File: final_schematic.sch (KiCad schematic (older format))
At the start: 49 parts, among them J1 Battery Babysitter, J2 BB_SYSOFF, J3 BOOT0, J4 OLED Qwiic, J5 Programmer, J8 GPS_COAX, SW1 SW_Push_SESS, SW2 SW_Push_RADIO, SW3 SW_Push_RST, U1 STM32L476VGTx, U2 MTK3339, U3 RFM95W-868S2, U4 BNO055, U5 LT1129-3.3_SO8

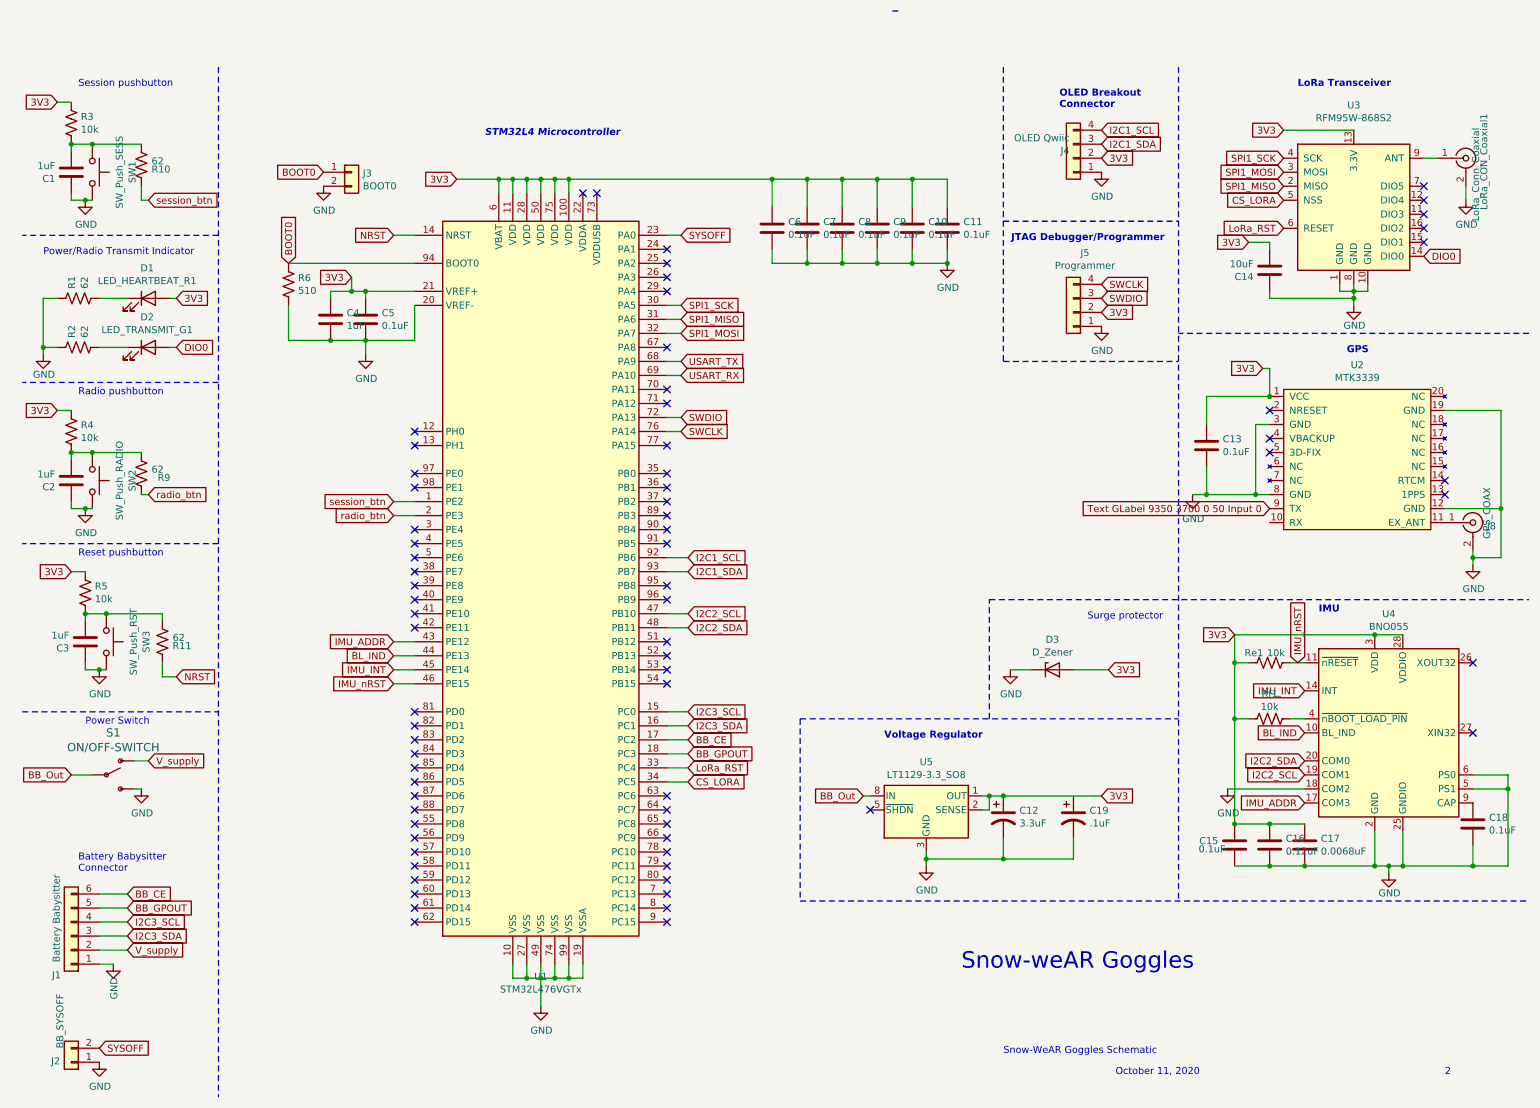
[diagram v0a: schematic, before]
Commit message: Schematic FINAL 	modified:   final_schematic-cache.lib 	modified:   final_schematic.sch 	modified:   final_schematic.sch-bak
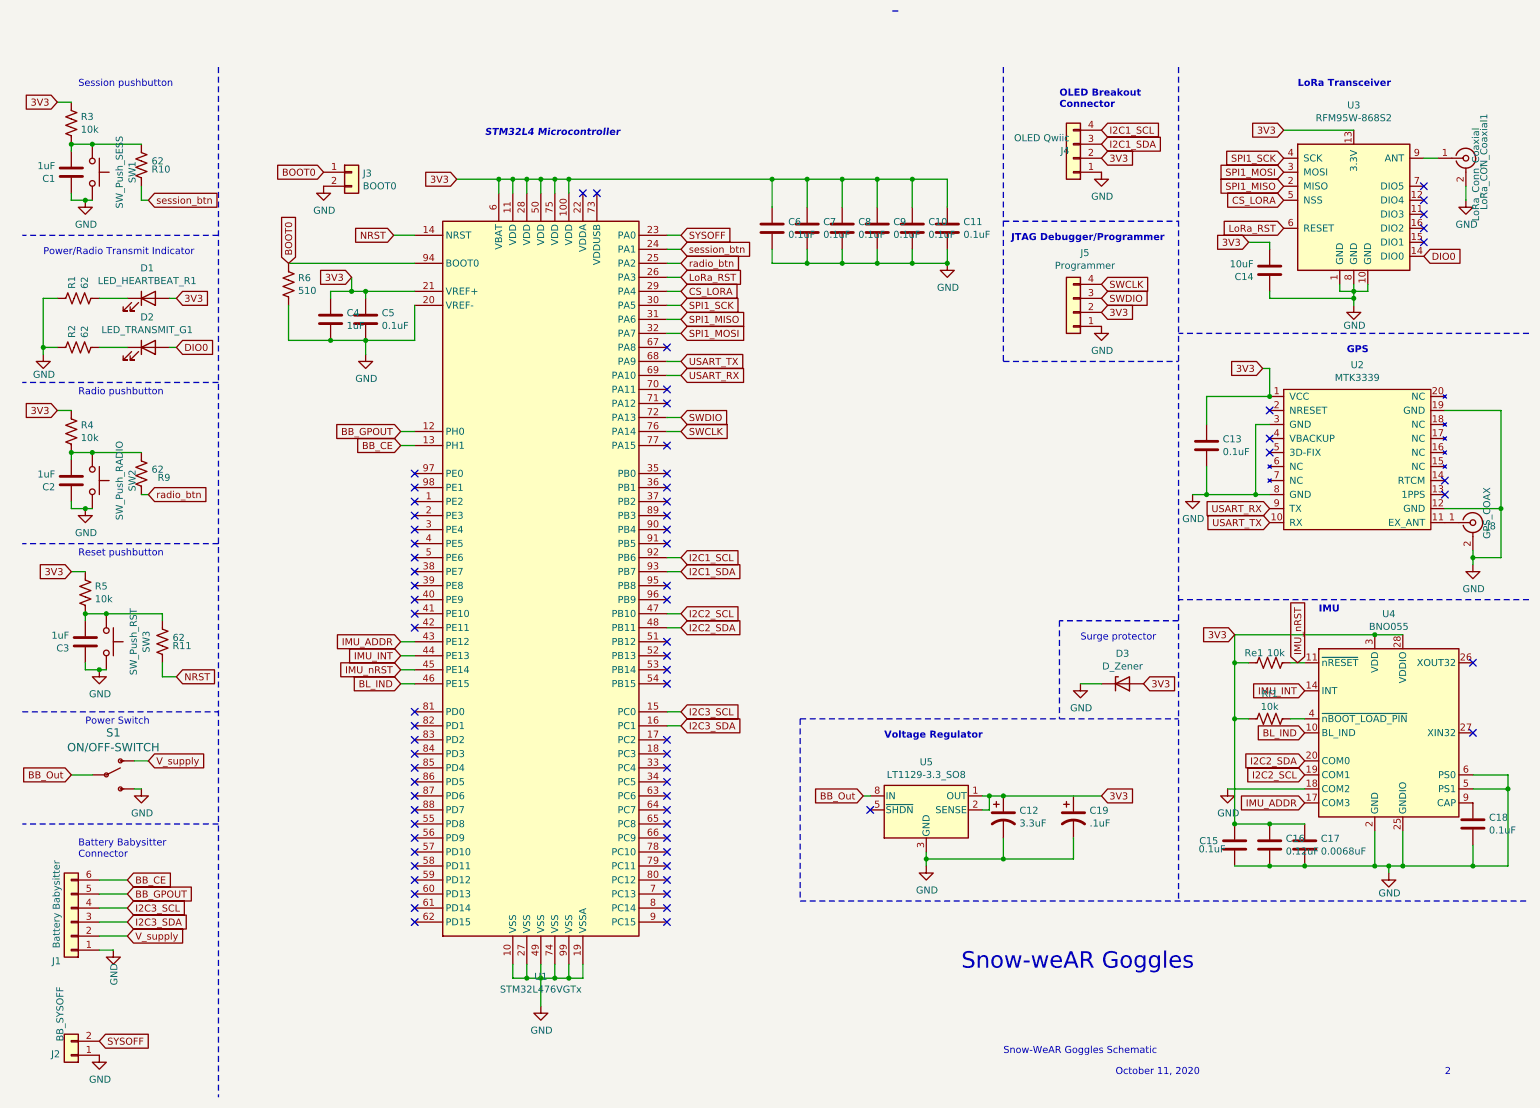
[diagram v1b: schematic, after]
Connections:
- net Text GLabel 9350 3700 0    50   Input ~ 0 is gone; now on net USART_RX: U2.9 (TX)
- net BB_CE: now also U1.13 (PH1); no longer U1.17 (PC2)
- net BB_GPOUT: now also U1.12 (PH0); no longer U1.18 (PC3)
- net BL_IND: now also U1.46 (PE15); no longer U1.44 (PE13)
- net CS_LORA: now also U1.29 (PA4); no longer U1.34 (PC5)
- net IMU_INT: now also U1.44 (PE13); no longer U1.45 (PE14)
- net IMU_nRST: now also U1.45 (PE14); no longer U1.46 (PE15)
- net LoRa_RST: now also U1.26 (PA3); no longer U1.33 (PC4)
- net USART_TX: now also U2.10 (RX)
- net radio_btn: now also U1.25 (PA2); no longer U1.2 (PE3)
- net session_btn: now also U1.24 (PA1); no longer U1.1 (PE2)
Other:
- moved on the sheet: D3, J1, J2
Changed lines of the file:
@@
 EESchema Schematic File Version 4
-LIBS:final_schematic-cache
-EELAYER 26 0
+EELAYER 30 0
 EELAYER END
 $Descr A4 11693 8268
@@
 $EndComp
 Text GLabel 9350 3600 0    50   Input ~ 0
-Text GLabel 9350 3700 0    50   Input ~ 0
-USART_TX
+USART_RX
 $Comp
 L final_schematic-rescue:MTK3339-GPS-rescue U2
@@
 L Connector_Generic:Conn_01x06 J1
 U 1 1 5FF26B1F
-P 800 6650
-F 0 "J1" H 906 6928 50  0000 C CNN
-F 1 "Battery Babysitter" V 906 6837 50  0000 R CNN
-F 2 "Connector_PinHeader_1.00mm:PinHeader_1x06_P1.00mm_Vertical" H 800 6650 50  0001 C CNN
-F 3 "~" H 800 6650 50  0001 C CNN
-	1    800  6650
+P 800 6550
+F 0 "J1" H 906 6828 50  0000 C CNN
+F 1 "Battery Babysitter" V 906 6737 50  0000 R CNN
+F 2 "Connector_PinHeader_1.00mm:PinHeader_1x06_P1.00mm_Vertical" H 800 6550 50  0001 C CNN
+F 3 "~" H 800 6550 50  0001 C CNN
+	1    800  6550
 	-1   0    0    1
 $EndComp
-Text Notes 850  6200 0    50   ~ 0
+Text Notes 850  6100 0    50   ~ 0
 Battery Babysitter \nConnector
+Text GLabel 1200 6550 2    50   Input ~ 0
+I2C3_SDA
+Text GLabel 1200 6450 2    50   Input ~ 0
+I2C3_SCL
 Text GLabel 1200 6650 2    50   Input ~ 0
-I2C3_SDA
-Text GLabel 1200 6550 2    50   Input ~ 0
-I2C3_SCL
-Text GLabel 1200 6750 2    50   Input ~ 0
 V_supply
 Wire Wire Line
-	1200 6750 1000 6750
-Wire Wire Line
 	1200 6650 1000 6650
+Wire Wire Line
+	1200 6550 1000 6550
 $Comp
 L power:GND #PWR05
 U 1 1 60007EB3
-P 1100 6850
-F 0 "#PWR05" H 1100 6600 50  0001 C CNN
-F 1 "GND" V 1105 6677 50  0000 C CNN
-F 2 "" H 1100 6850 50  0001 C CNN
-F 3 "" H 1100 6850 50  0001 C CNN
-	1    1100 6850
-	1    0    0    -1
-$EndComp
-Wire Wire Line
-	1200 6550 1000 6550
+P 1100 6750
+F 0 "#PWR05" H 1100 6500 50  0001 C CNN
+F 1 "GND" V 1105 6577 50  0000 C CNN
+F 2 "" H 1100 6750 50  0001 C CNN
+F 3 "" H 1100 6750 50  0001 C CNN
+	1    1100 6750
+	1    0    0    -1
+$EndComp
+Wire Wire Line
+	1200 6450 1000 6450
 Text Notes 8600 1700 2    50   ~ 10
 JTAG Debugger/Programmer
@@
 Text GLabel 9600 5500 0    50   Input ~ 0
 I2C2_SCL
-Text GLabel 1200 6450 2    50   Input ~ 0
+Text GLabel 1200 6350 2    50   Input ~ 0
 BB_GPOUT
 Wire Wire Line
-	1000 6350 1200 6350
-Wire Wire Line
-	1200 6450 1000 6450
+	1000 6250 1200 6250
+Wire Wire Line
+	1200 6350 1000 6350
 NoConn ~ 10600 3400
 NoConn ~ 10600 3500
@@
 Text GLabel 2800 1950 0    50   Input ~ 0
 3V3
-Text GLabel 3100 4650 0    50   Input ~ 0
+Text GLabel 3150 4850 0    50   Input ~ 0
 BL_IND
-Text GLabel 3100 4550 0    50   Input ~ 0
+Text GLabel 3150 4550 0    50   Input ~ 0
 IMU_ADDR
 Text GLabel 2600 1200 0    50   Input ~ 0
@@
 Text GLabel 5150 1650 2    50   Input ~ 0
 SYSOFF
-Text GLabel 5200 5350 2    50   Input ~ 0
+Text GLabel 3150 3050 0    50   Input ~ 0
 BB_GPOUT
-Text GLabel 3100 4850 0    50   Input ~ 0
+Text GLabel 3150 4750 0    50   Input ~ 0
 IMU_nRST
 NoConn ~ 3250 3450
@@
 NoConn ~ 5050 2850
 NoConn ~ 5050 2750
-NoConn ~ 5050 1850
-NoConn ~ 5050 1750
 NoConn ~ 4550 1350
 NoConn ~ 4450 1350
@@
 NoConn ~ 3250 3850
 NoConn ~ 3250 3750
-Text GLabel 3100 3550 0    50   Input ~ 0
+Text GLabel 5150 1750 2    50   Input ~ 0
 session_btn
-Text GLabel 3100 3650 0    50   Input ~ 0
+Text GLabel 5150 1850 2    50   Input ~ 0
 radio_btn
 Wire Wire Line
@@
 	4250 1250 4350 1250
 Connection ~ 4150 1250
-Text GLabel 3100 4750 0    50   Input ~ 0
+Text GLabel 3150 4650 0    50   Input ~ 0
 IMU_INT
-Text GLabel 5200 5550 2    50   Input ~ 0
+Text GLabel 5150 2050 2    50   Input ~ 0
 CS_LORA
-Text GLabel 5200 5450 2    50   Input ~ 0
+Text GLabel 5150 1950 2    50   Input ~ 0
 LoRa_RST
-Text GLabel 5200 5250 2    50   Input ~ 0
+Text GLabel 3150 3150 0    50   Input ~ 0
 BB_CE
-Text GLabel 5200 4450 2    50   Input ~ 0
+Text GLabel 5150 4450 2    50   Input ~ 0
 I2C2_SDA
-Text GLabel 5200 4350 2    50   Input ~ 0
+Text GLabel 5150 4350 2    50   Input ~ 0
 I2C2_SCL
 Connection ~ 4350 6950
@@
 Wire Wire Line
 	9050 5600 9600 5600
-Text GLabel 1200 6350 2    50   Input ~ 0
+Text GLabel 1200 6250 2    50   Input ~ 0
 BB_CE
 Wire Wire Line
@@
 L Connector_Generic:Conn_01x02 J2
 U 1 1 5FC7E508
-P 800 7550
-F 0 "J2" H 880 7542 50  0000 L CNN
-F 1 "BB_SYSOFF" V 880 7451 50  0000 R CNN
-F 2 "Connector_PinHeader_1.00mm:PinHeader_1x02_P1.00mm_Vertical" H 800 7550 50  0001 C CNN
-F 3 "~" H 800 7550 50  0001 C CNN
-	1    800  7550
+P 800 7500
+F 0 "J2" H 880 7492 50  0000 L CNN
+F 1 "BB_SYSOFF" V 880 7401 50  0000 R CNN
+F 2 "Connector_PinHeader_1.00mm:PinHeader_1x02_P1.00mm_Vertical" H 800 7500 50  0001 C CNN
+F 3 "~" H 800 7500 50  0001 C CNN
+	1    800  7500
 	-1   0    0    1
 $EndComp
@@
 L power:GND #PWR?
 U 1 1 5FC7E50E
-P 1000 7550
+P 1000 7500
 AR Path="/5F775B0B/5FC7E50E" Ref="#PWR?"  Part="1"
 AR Path="/5FC7E50E" Ref="#PWR0104"  Part="1"
-F 0 "#PWR0104" H 1000 7300 50  0001 C CNN
-F 1 "GND" H 1005 7377 50  0000 C CNN
-F 2 "" H 1000 7550 50  0001 C CNN
-F 3 "" H 1000 7550 50  0001 C CNN
-	1    1000 7550
-	1    0    0    -1
-$EndComp
-Text GLabel 1000 7450 2    50   Input ~ 0
+F 0 "#PWR0104" H 1000 7250 50  0001 C CNN
+F 1 "GND" H 1005 7327 50  0000 C CNN
+F 2 "" H 1000 7500 50  0001 C CNN
+F 3 "" H 1000 7500 50  0001 C CNN
+	1    1000 7500
+	1    0    0    -1
+$EndComp
+Text GLabel 1000 7400 2    50   Input ~ 0
 SYSOFF
 $Comp
@@
 NoConn ~ 6500 5750
 NoConn ~ 9350 3200
-NoConn ~ 5050 2050
 NoConn ~ 5050 2450
 NoConn ~ 5050 3650
 Wire Wire Line
-	1100 6850 1000 6850
+	1100 6750 1000 6750
 Wire Wire Line
 	7300 5750 7350 5750
@@
 	600  2450 600  2500
 Connection ~ 600  2450
-Text GLabel 5200 4050 2    50   Input ~ 0
+Text GLabel 5150 4050 2    50   Input ~ 0
 I2C1_SDA
-Text GLabel 5200 3950 2    50   Input ~ 0
+Text GLabel 5150 3950 2    50   Input ~ 0
 I2C1_SCL
-Text GLabel 5200 5150 2    50   Input ~ 0
+Text GLabel 5150 5150 2    50   Input ~ 0
 I2C3_SDA
-Text GLabel 5200 5050 2    50   Input ~ 0
+Text GLabel 5150 5050 2    50   Input ~ 0
 I2C3_SCL
 Wire Wire Line
@@
 Wire Wire Line
 	5050 3050 5150 3050
-Wire Wire Line
-	5200 3950 5050 3950
-Wire Wire Line
-	5050 4050 5200 4050
-Wire Wire Line
-	5200 4350 5050 4350
-Wire Wire Line
-	5050 4450 5200 4450
-Wire Wire Line
-	5200 5050 5050 5050
-Wire Wire Line
-	5050 5150 5200 5150
-Wire Wire Line
-	5200 5250 5050 5250
-Wire Wire Line
-	5200 5350 5050 5350
-Wire Wire Line
-	5200 5450 5050 5450
-Wire Wire Line
-	5200 5550 5050 5550
-Wire Wire Line
-	3100 3550 3250 3550
-Wire Wire Line
-	3250 3650 3100 3650
-Wire Wire Line
-	3100 4550 3250 4550
-Wire Wire Line
-	3250 4650 3100 4650
-Wire Wire Line
-	3100 4750 3250 4750
-Wire Wire Line
-	3250 4850 3100 4850
 Wire Wire Line
 	4350 1250 5800 1250
 Connection ~ 4350 1250
-NoConn ~ 5050 1950
 NoConn ~ 5050 3350
 NoConn ~ 5050 3450
-NoConn ~ 3250 3050
-NoConn ~ 3250 3150
 NoConn ~ 3250 3350
 NoConn ~ 5050 4550
@@
 L Device:D_Zener D3
 U 1 1 5F894344
-P 7800 4750
-F 0 "D3" H 7800 4966 50  0000 C CNN
-F 1 "D_Zener" H 7800 4875 50  0000 C CNN
-F 2 "footprint_lib:1N5355BRLG" H 7800 4750 50  0001 C CNN
-F 3 "~" H 7800 4750 50  0001 C CNN
-	1    7800 4750
-	1    0    0    -1
-$EndComp
-Text GLabel 8200 4750 2    50   Input ~ 0
+P 8300 4850
+F 0 "D3" H 8300 5066 50  0000 C CNN
+F 1 "D_Zener" H 8300 4975 50  0000 C CNN
+F 2 "footprint_lib:1N5355BRLG" H 8300 4850 50  0001 C CNN
+F 3 "~" H 8300 4850 50  0001 C CNN
+	1    8300 4850
+	1    0    0    -1
+$EndComp
+Text GLabel 8450 4850 2    50   Input ~ 0
 3V3
 $Comp
 L power:GND #PWR010
 U 1 1 5F8944C0
-P 7500 4750
-F 0 "#PWR010" H 7500 4500 50  0001 C CNN
-F 1 "GND" H 7505 4577 50  0000 C CNN
-F 2 "" H 7500 4750 50  0001 C CNN
-F 3 "" H 7500 4750 50  0001 C CNN
-	1    7500 4750
-	1    0    0    -1
-$EndComp
-Wire Wire Line
-	7650 4750 7500 4750
-Wire Wire Line
-	8200 4750 7950 4750
+P 8000 4850
+F 0 "#PWR010" H 8000 4600 50  0001 C CNN
+F 1 "GND" H 8005 4677 50  0000 C CNN
+F 2 "" H 8000 4850 50  0001 C CNN
+F 3 "" H 8000 4850 50  0001 C CNN
+	1    8000 4850
+	1    0    0    -1
+$EndComp
+Wire Wire Line
+	8150 4850 8000 4850
 $Comp
 L Device:CP1 C19
@@
 Wire Notes Line
 	6000 6400 11200 6400
-Wire Notes Line
-	7350 5100 7350 4250
-Wire Notes Line
-	7350 4250 11200 4250
-Text Notes 8050 4400 0    50   ~ 0
+Text Notes 8000 4550 0    50   ~ 0
 Surge protector
+Text GLabel 9350 3700 0    50   Input ~ 0
+USART_TX
+Wire Notes Line
+	11200 4250 8700 4250
+Wire Notes Line
+	8700 4400 7850 4400
+Wire Notes Line
+	7850 4400 7850 5100
+Wire Notes Line
+	1850 5850 450  5850
+Wire Wire Line
+	5050 1750 5150 1750
+Wire Wire Line
+	5050 1850 5150 1850
+Wire Wire Line
+	5050 1950 5150 1950
+Wire Wire Line
+	5050 2050 5150 2050
+Wire Wire Line
+	5150 3950 5050 3950
+Wire Wire Line
+	5050 4050 5150 4050
+Wire Wire Line
+	5150 4350 5050 4350
+Wire Wire Line
+	5050 4450 5150 4450
+Wire Wire Line
+	5150 5050 5050 5050
+Wire Wire Line
+	5050 5150 5150 5150
+Wire Wire Line
+	3250 4550 3150 4550
+Wire Wire Line
+	3150 4650 3250 4650
+Wire Wire Line
+	3250 4750 3150 4750
+Wire Wire Line
+	3150 4850 3250 4850
+Wire Wire Line
+	3250 3050 3150 3050
+Wire Wire Line
+	3150 3150 3250 3150
+NoConn ~ 5050 5250
+NoConn ~ 5050 5350
+NoConn ~ 5050 5450
+NoConn ~ 5050 5550
+NoConn ~ 3250 3550
+NoConn ~ 3250 3650
 $EndSCHEMATC

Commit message: Please be right
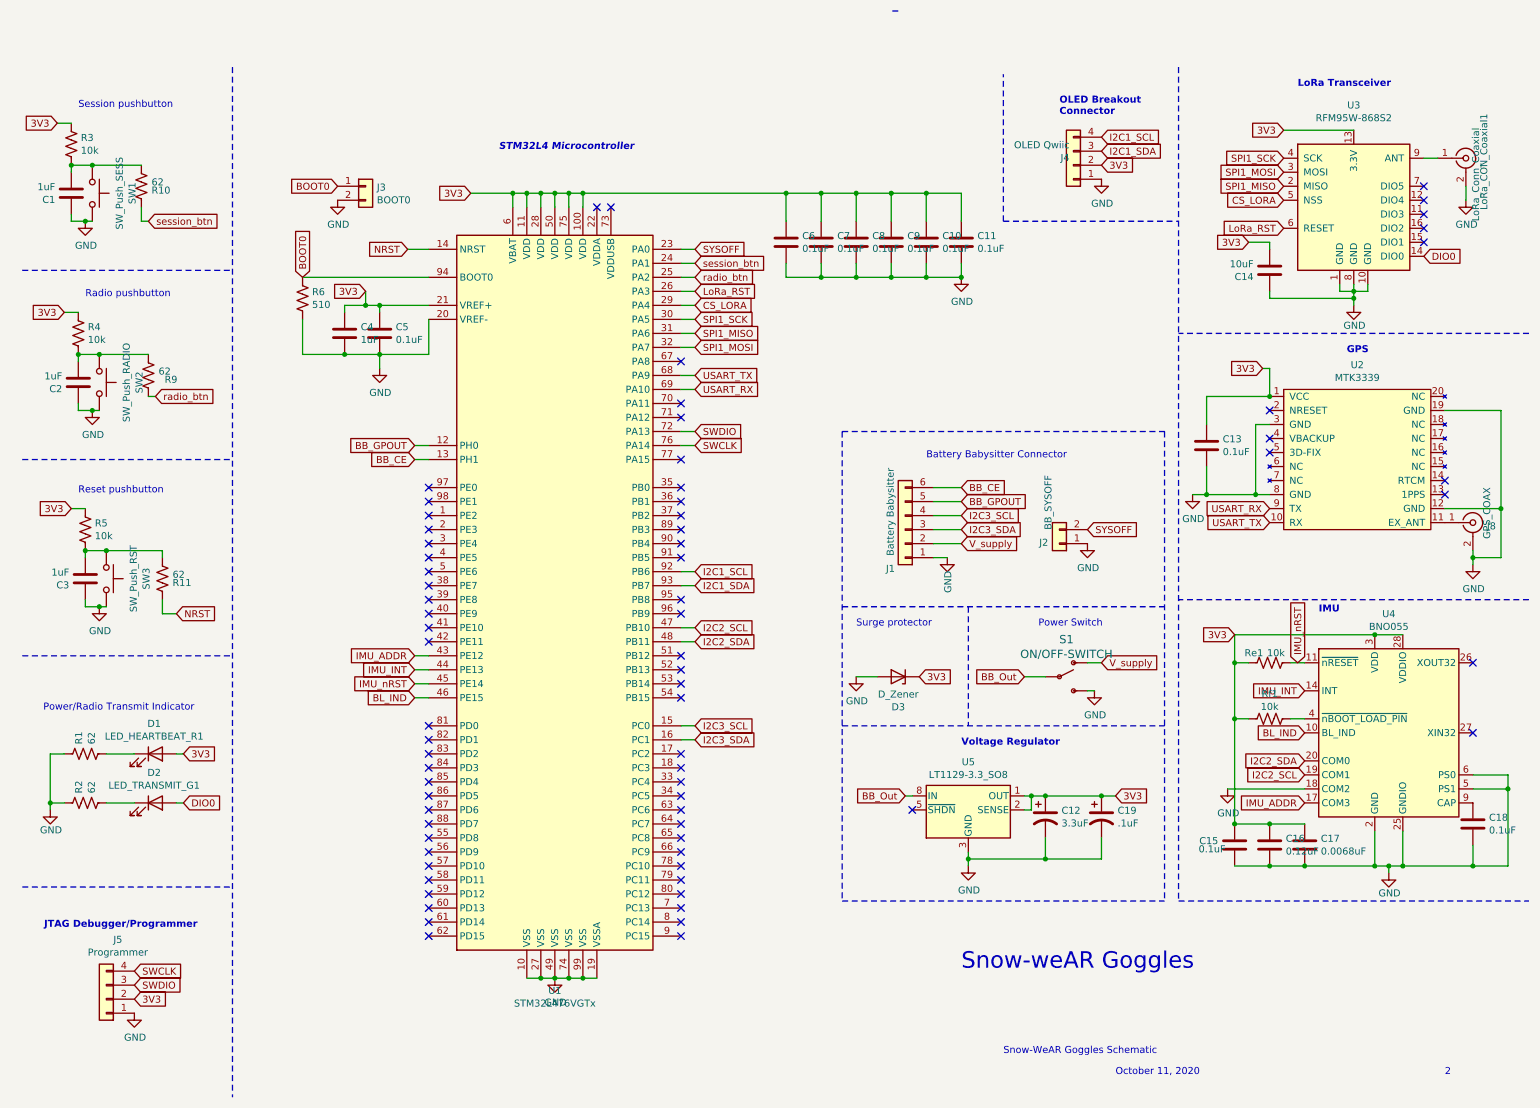
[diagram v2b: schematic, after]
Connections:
- net 3V3: now also C19.1, D3.1 (K); no longer D3.2 (A)
- net GND: now also D3.2 (A); no longer D3.1 (K)
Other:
- note added: "Battery Babysitter Connector"
- note removed: "Battery Babysitter \nConnector"
- moved on the sheet: C1, C10, C11, C12, C19, C2, C3, C4, C5, C6, C7, C8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
